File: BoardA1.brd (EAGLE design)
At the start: 44 x 100.5 mm, 20 parts, among them J1 LOAD_CELL1X03-PTH, J2 FEMALE 2x3, J3 LOAD_CELL1X03-PTH, J5 LOAD_CELL1X03-PTH, J6 LOAD_CELL1X03-PTH

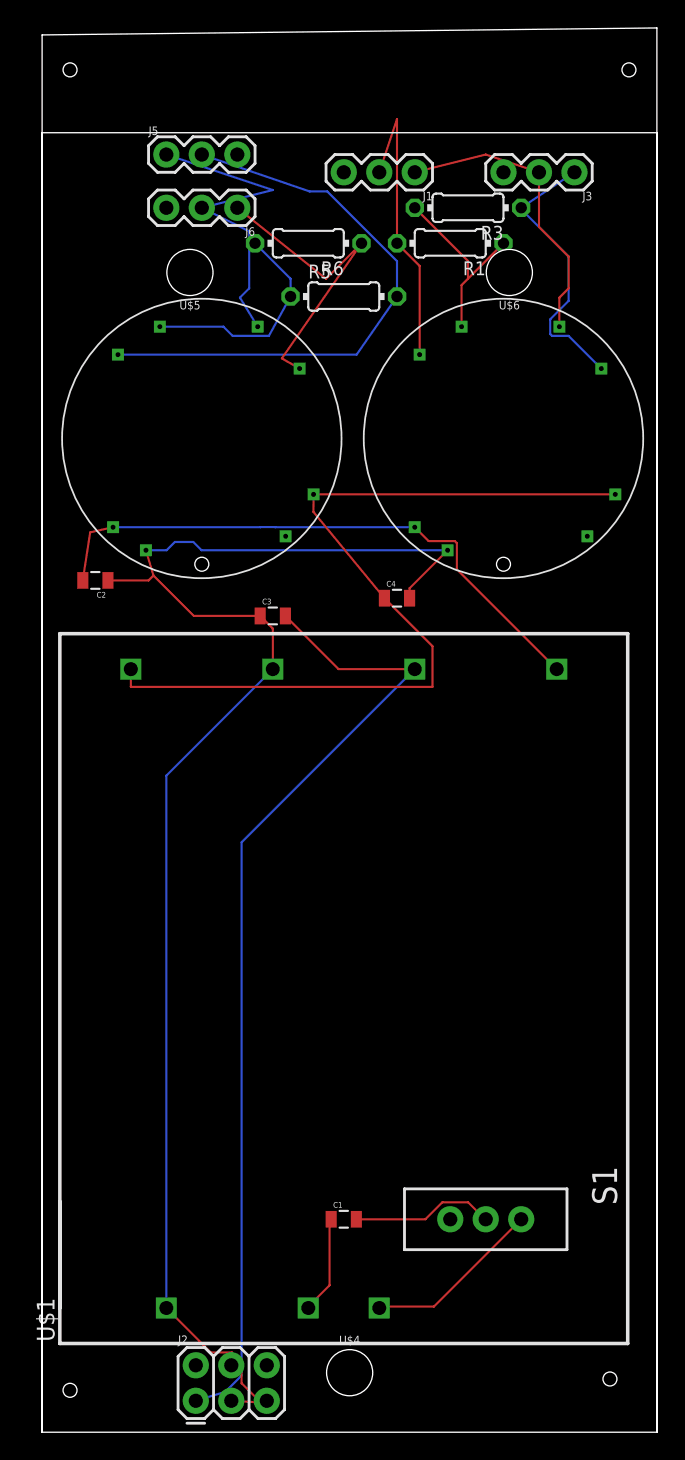
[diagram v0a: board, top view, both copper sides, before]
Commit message: Merge branch 'master' of https://github.com/Luckycyq1010/SmartCrutch-ProtoBeta
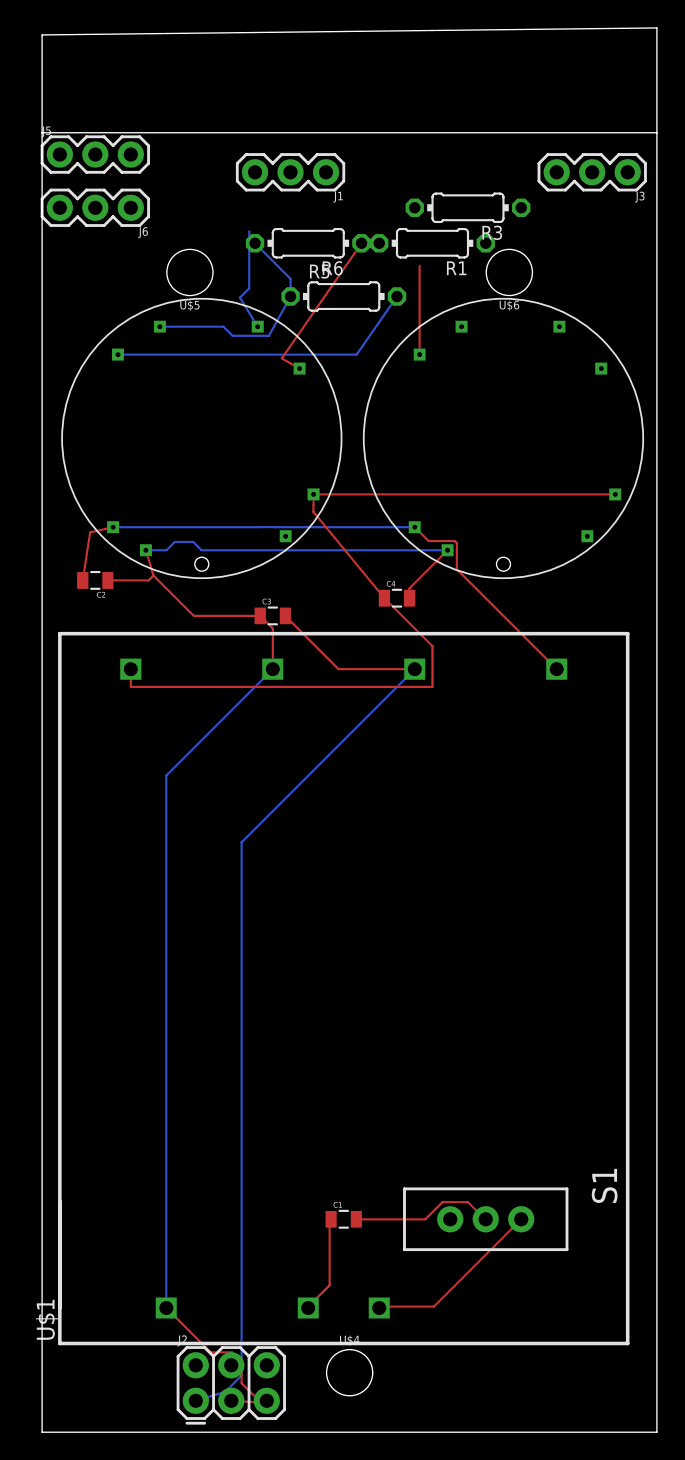
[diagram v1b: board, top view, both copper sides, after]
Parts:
- moved J5 7.62 mm to (1.27, 91.4)
- moved J6 7.62 mm to (6.35, 87.6)
- moved J1 6.35 mm to (20.3, 90.2)
- moved J3 3.81 mm to (41.9, 90.2)
- moved R1 1.27 mm to (27.9, 85.1)
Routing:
- net -SIG1: track 21.5 -> 0.00 mm
- net -EX1: track 20.4 -> 0.12 mm
- net +EX2: track 41.1 -> 22.1 mm
- net -SIG2: track 24.5 -> 7.45 mm
- net +EX1: track 21.5 -> 6.35 mm
- net +SIG1: track 13.9 -> 0.00 mm
- net -EX2: track 23.2 -> 11.5 mm
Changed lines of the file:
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@@
 <plain>
 <wire x1="0" y1="0" x2="44" y2="0" width="0" layer="20"/>
-<wire x1="44" y1="0" x2="44" y2="100.5" width="0" layer="20"/>
+<wire x1="44" y1="93" x2="44" y2="100.5" width="0" layer="20"/>
 <wire x1="44" y1="100.5" x2="0" y2="100" width="0" layer="20"/>
-<wire x1="0" y1="100" x2="0" y2="0" width="0" layer="20"/>
-<hole x="2" y="3" drill="1"/>
-<hole x="40.64" y="3.81" drill="1"/>
-<hole x="42" y="97.5" drill="1"/>
-<hole x="2" y="97.5" drill="1"/>
+<wire x1="0" y1="100" x2="0" y2="93" width="0" layer="20"/>
 <dimension x1="0" y1="0" x2="44" y2="0" x3="22" y3="-3.81" textsize="1.778" layer="1"/>
 <dimension x1="44" y1="0" x2="44" y2="100.5" x3="48.26" y3="50.25" textsize="1.778" layer="1"/>
@@
 <element name="C3" library="SparkFun-Capacitors" package="0805" value="" x="16.51" y="58.42"/>
 <element name="C4" library="SparkFun-Capacitors" package="0805" value="" x="25.4" y="59.69"/>
-<element name="J1" library="Smartcrutches" package="1X03" value="LOAD_CELL1X03-PTH" x="26.67" y="90.17" rot="R180">
-<attribute name="SF_ID" value="SEN-10245" x="26.67" y="90.17" size="1.778" layer="27" rot="R180" display="off"/>
-</element>
-<element name="J3" library="Smartcrutches" package="1X03" value="LOAD_CELL1X03-PTH" x="38.1" y="90.17" rot="R180">
-<attribute name="SF_ID" value="SEN-10245" x="38.1" y="90.17" size="1.778" layer="27" rot="R180" display="off"/>
-</element>
-<element name="J5" library="Smartcrutches" package="1X03" value="LOAD_CELL1X03-PTH" x="8.89" y="91.44">
-<attribute name="SF_ID" value="SEN-10245" x="8.89" y="91.44" size="1.778" layer="27" display="off"/>
-</element>
-<element name="J6" library="Smartcrutches" package="1X03" value="LOAD_CELL1X03-PTH" x="13.97" y="87.63" rot="R180">
-<attribute name="SF_ID" value="SEN-10245" x="13.97" y="87.63" size="1.778" layer="27" rot="R180" display="off"/>
-</element>
-<element name="R1" library="eagle-ltspice" library_urn="urn:adsk.eagle:library:217" package="0204/7" value="" x="29.21" y="85.09" rot="R180">
-<attribute name="SPICEMODEL" value="NONE" x="29.21" y="85.09" size="1.778" layer="27" rot="R180" display="off"/>
-<attribute name="SPICEPREFIX" value="R" x="29.21" y="85.09" size="1.778" layer="27" rot="R180" display="off"/>
+<element name="J1" library="Smartcrutches" package="1X03" value="LOAD_CELL1X03-PTH" x="20.32" y="90.17" rot="R180">
+<attribute name="SF_ID" value="SEN-10245" x="20.32" y="90.17" size="1.778" layer="27" rot="R180" display="off"/>
+</element>
+<element name="J3" library="Smartcrutches" package="1X03" value="LOAD_CELL1X03-PTH" x="41.91" y="90.17" rot="R180">
+<attribute name="SF_ID" value="SEN-10245" x="41.91" y="90.17" size="1.778" layer="27" rot="R180" display="off"/>
+</element>
+<element name="J5" library="Smartcrutches" package="1X03" value="LOAD_CELL1X03-PTH" x="1.27" y="91.44">
+<attribute name="SF_ID" value="SEN-10245" x="1.27" y="91.44" size="1.778" layer="27" display="off"/>
+</element>
+<element name="J6" library="Smartcrutches" package="1X03" value="LOAD_CELL1X03-PTH" x="6.35" y="87.63" rot="R180">
+<attribute name="SF_ID" value="SEN-10245" x="6.35" y="87.63" size="1.778" layer="27" rot="R180" display="off"/>
+</element>
+<element name="R1" library="eagle-ltspice" library_urn="urn:adsk.eagle:library:217" package="0204/7" value="" x="27.94" y="85.09" rot="R180">
+<attribute name="SPICEMODEL" value="NONE" x="27.94" y="85.09" size="1.778" layer="27" rot="R180" display="off"/>
+<attribute name="SPICEPREFIX" value="R" x="27.94" y="85.09" size="1.778" layer="27" rot="R180" display="off"/>
 </element>
 <element name="R3" library="eagle-ltspice" library_urn="urn:adsk.eagle:library:217" package="0204/7" value="" x="30.48" y="87.63" rot="R180">
@@
 <contactref element="J3" pad="1"/>
 <wire x1="39.9288" y1="76.2" x2="40.02" y2="76.12" width="0.1524" layer="1"/>
-<wire x1="38.1" y1="90.17" x2="34.29" y2="87.63" width="0.1524" layer="16"/>
-<wire x1="36.3624" y1="79.6436875" x2="36.3624" y2="78.5963125" width="0.1524" layer="16"/>
-<wire x1="36.3624" y1="78.5963125" x2="36.4963125" y2="78.4624" width="0.1524" layer="16"/>
-<wire x1="34.29" y1="87.63" x2="34.29" y2="87.529475" width="0.1524" layer="16"/>
-<wire x1="37.6776" y1="78.4624" x2="40.02" y2="76.12" width="0.1524" layer="16"/>
-<wire x1="34.29" y1="87.529475" x2="37.6832" y2="84.136275" width="0.1524" layer="16"/>
-<wire x1="36.4963125" y1="78.4624" x2="37.6776" y2="78.4624" width="0.1524" layer="16"/>
-<wire x1="37.6832" y1="84.136275" x2="37.6832" y2="80.9644875" width="0.1524" layer="16"/>
-<wire x1="37.6832" y1="80.9644875" x2="36.3624" y2="79.6436875" width="0.1524" layer="16"/>
+<wire x1="34.29" y1="87.63" x2="41.91" y2="90.17" width="0" layer="19" extent="1-1"/>
+<wire x1="39.9288" y1="76.2" x2="34.29" y2="87.63" width="0" layer="19" extent="1-1"/>
 </signal>
 <signal name="-SIG1">
@@
 <contactref element="J3" pad="2"/>
 <contactref element="J1" pad="1"/>
-<wire x1="26.67" y1="90.17" x2="31.75" y2="91.44" width="0.1524" layer="1"/>
-<wire x1="31.75" y1="91.44" x2="35.56" y2="90.17" width="0.1524" layer="1"/>
-<wire x1="37.6832" y1="84.136275" x2="37.6832" y2="81.863725" width="0.1524" layer="1"/>
-<wire x1="35.56" y1="90.17" x2="35.56" y2="86.259475" width="0.1524" layer="1"/>
-<wire x1="37.6832" y1="81.863725" x2="37.02" y2="81.200525" width="0.1524" layer="1"/>
-<wire x1="37.02" y1="81.200525" x2="37.02" y2="79.12" width="0.1524" layer="1"/>
-<wire x1="35.56" y1="86.259475" x2="37.6832" y2="84.136275" width="0.1524" layer="1"/>
+<wire x1="37.02" y1="79.12" x2="39.37" y2="90.17" width="0" layer="19" extent="1-1"/>
+<wire x1="20.32" y1="90.17" x2="39.37" y2="90.17" width="0" layer="19" extent="1-1"/>
 </signal>
 <signal name="+SIG1">
@@
 <contactref element="R3" pad="2"/>
 <contactref element="R1" pad="1"/>
-<wire x1="30.02" y1="82.09" x2="30.02" y2="79.12" width="0.1524" layer="1"/>
-<wire x1="33.02" y1="85.09" x2="30.48" y2="82.55" width="0.1524" layer="1"/>
-<wire x1="30.48" y1="82.55" x2="30.02" y2="82.09" width="0.1524" layer="1"/>
-<wire x1="30.48" y1="82.55" x2="30.48" y2="83.82" width="0.1524" layer="1"/>
-<wire x1="30.48" y1="83.82" x2="26.67" y2="87.63" width="0.1524" layer="1"/>
+<wire x1="30.02" y1="79.12" x2="31.75" y2="85.09" width="0" layer="19" extent="1-1"/>
+<wire x1="26.67" y1="87.63" x2="31.75" y2="85.09" width="0" layer="19" extent="1-1"/>
 </signal>
 <signal name="+EX1">
@@
 <contactref element="J1" pad="2"/>
 <wire x1="27.02" y1="77.12" x2="27.02" y2="83.47" width="0.1524" layer="1"/>
-<wire x1="27.02" y1="83.47" x2="25.4" y2="85.09" width="0.1524" layer="1"/>
-<wire x1="25.4" y1="85.09" x2="25.4" y2="93.98" width="0.1524" layer="1"/>
-<wire x1="25.4" y1="93.98" x2="24.13" y2="90.17" width="0.1524" layer="1"/>
+<wire x1="27.02" y1="83.47" x2="24.13" y2="85.09" width="0" layer="19" extent="1-16"/>
+<wire x1="24.13" y1="85.09" x2="17.78" y2="90.17" width="0" layer="19" extent="1-1"/>
 </signal>
 <signal name="-EX2">
@@
 <wire x1="18.43" y1="76.12" x2="17.16" y2="76.85" width="0.1524" layer="1"/>
 <wire x1="17.16" y1="76.85" x2="22.86" y2="85.09" width="0.1524" layer="1"/>
-<wire x1="22.86" y1="85.09" x2="20.32" y2="82.55" width="0.1524" layer="1"/>
-<wire x1="20.32" y1="82.55" x2="13.97" y2="87.63" width="0.1524" layer="1"/>
+<wire x1="22.86" y1="85.09" x2="6.35" y2="87.63" width="0" layer="19" extent="1-1"/>
 </signal>
 <signal name="-SIG2">
@@
 <wire x1="15.43" y1="79.12" x2="14.16" y2="81.200525" width="0.1524" layer="16"/>
 <wire x1="14.16" y1="81.200525" x2="14.8232" y2="81.863725" width="0.1524" layer="16"/>
-<wire x1="14.8232" y1="85.9432" x2="11.43" y2="87.63" width="0.1524" layer="16"/>
+<wire x1="14.8232" y1="85.9432" x2="3.81" y2="87.63" width="0" layer="19" extent="1-16"/>
 <wire x1="14.8232" y1="81.863725" x2="14.8232" y2="85.9432" width="0.1524" layer="16"/>
-<wire x1="11.43" y1="87.63" x2="16.51" y2="88.9" width="0.1524" layer="16"/>
-<wire x1="16.51" y1="88.9" x2="8.89" y2="91.44" width="0.1524" layer="16"/>
+<wire x1="3.81" y1="87.63" x2="16.51" y2="88.9" width="0" layer="19" extent="1-16"/>
+<wire x1="16.51" y1="88.9" x2="1.27" y2="91.44" width="0" layer="19" extent="1-16"/>
 </signal>
 <signal name="+SIG2">
@@
 <wire x1="5.43" y1="77.12" x2="22.51" y2="77.12" width="0.1524" layer="16"/>
 <wire x1="22.51" y1="77.12" x2="25.4" y2="81.28" width="0.1524" layer="16"/>
-<wire x1="19.1516" y1="88.7984" x2="11.43" y2="91.44" width="0.1524" layer="16"/>
-<wire x1="25.4" y1="81.28" x2="25.4" y2="83.8072375" width="0.1524" layer="16"/>
-<wire x1="25.4" y1="83.8072375" x2="20.4088375" y2="88.7984" width="0.1524" layer="16"/>
-<wire x1="20.4088375" y1="88.7984" x2="19.1516" y2="88.7984" width="0.1524" layer="16"/>
+<wire x1="5.43" y1="77.12" x2="3.81" y2="91.44" width="0" layer="19" extent="1-1"/>
 </signal>
 <signal name="N$4">
